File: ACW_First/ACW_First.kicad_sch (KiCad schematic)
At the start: 18 parts, among them J1 Screw_Terminal_01x02, J10 Conn_01x04_Pin, J11 24VDC, J12 Conn_01x02_Pin, J13 Conn_01x04_Socket, J14 Conn_01x02_Pin, J2 Conn_01x03_Pin, J3 3.8VDC, J4 5VDC, J5 12VDC, J6 Screw_Terminal_01x02, J7 Screw_Terminal_01x04, J8 Conn_01x02_Pin, J9 Conn_01x03_Socket

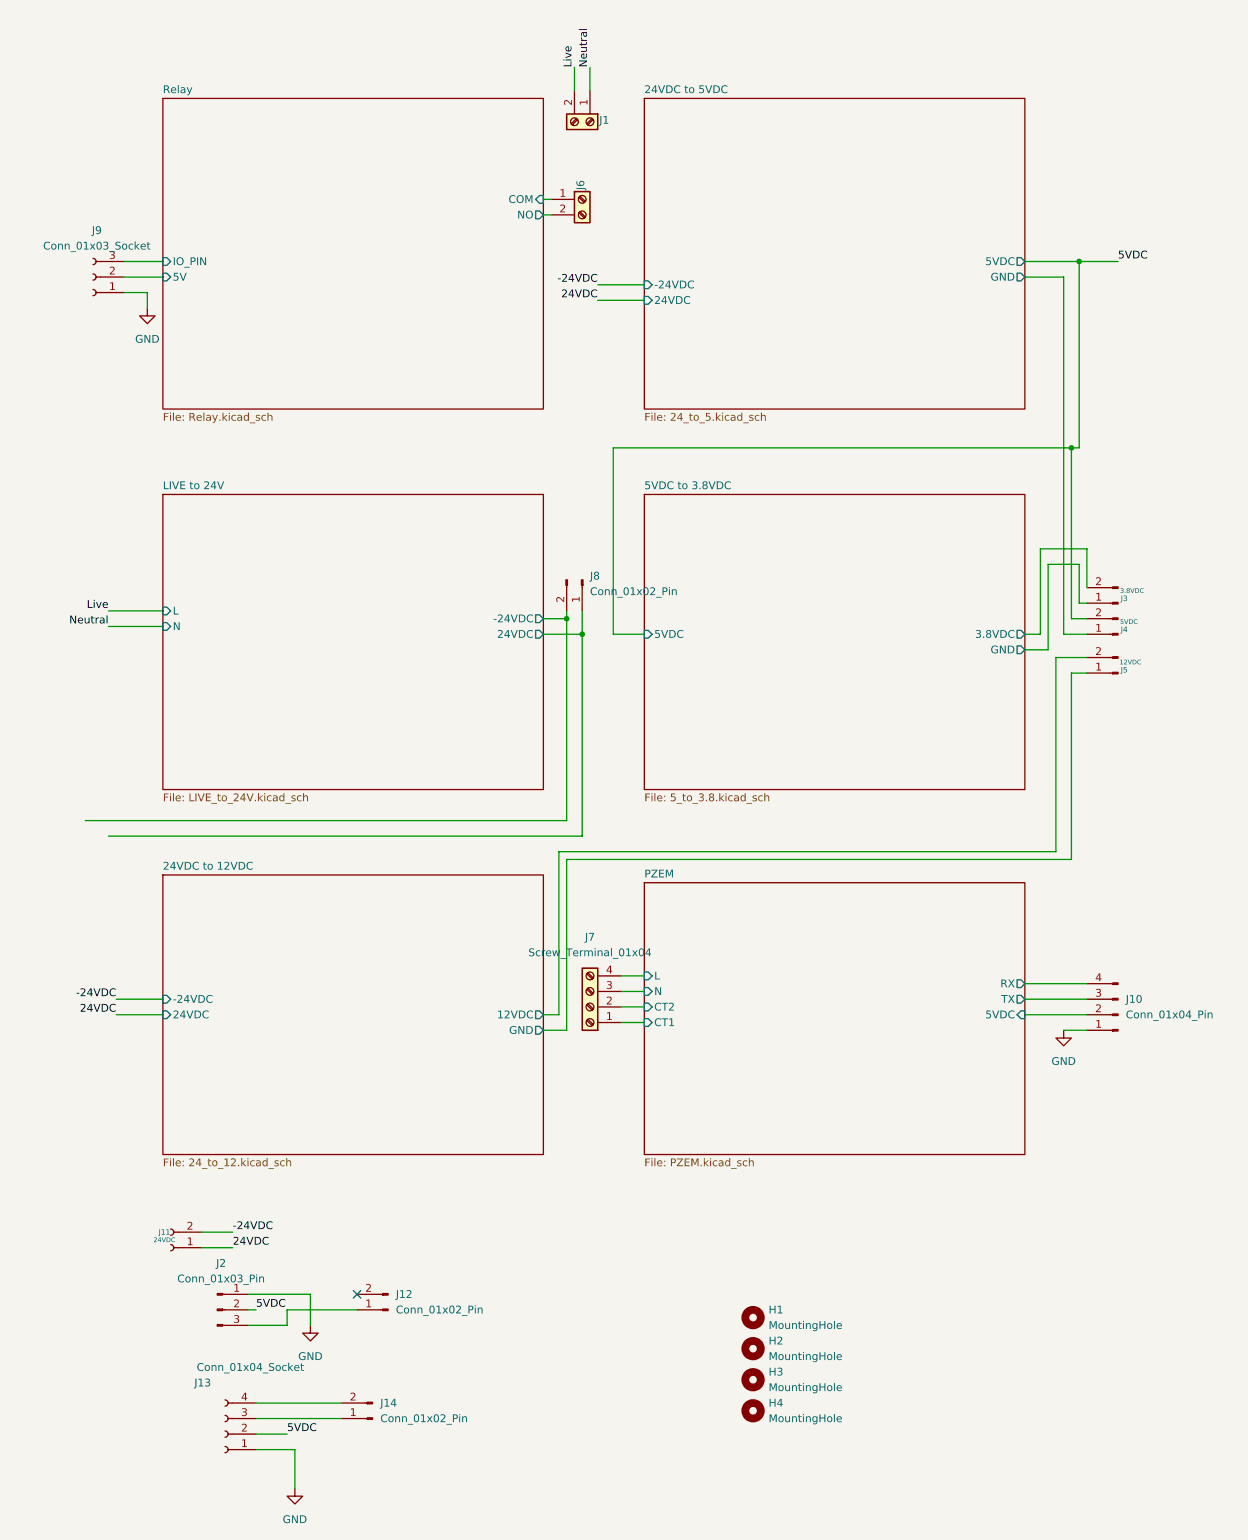
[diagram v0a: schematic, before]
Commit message: okokok
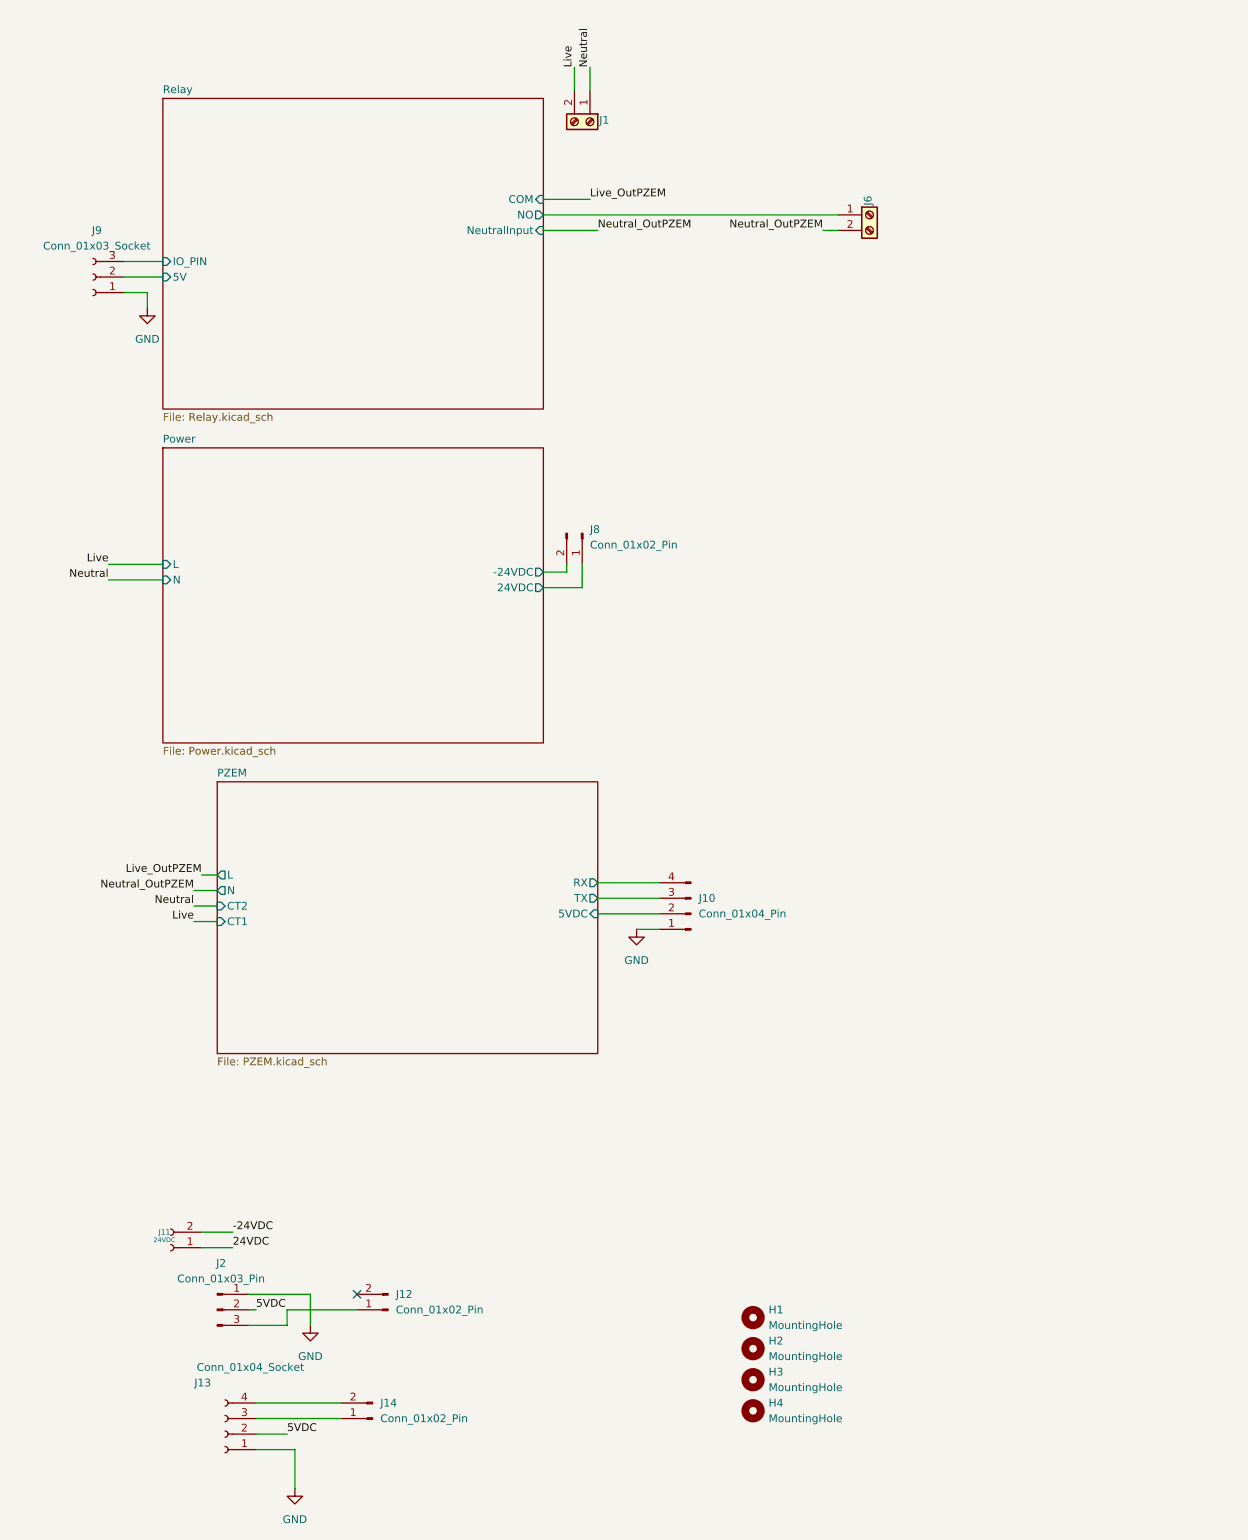
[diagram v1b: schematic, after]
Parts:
- removed J3: 3.8VDC, Connector_PinHeader_2.54mm:PinHeader_1x02_P2.54mm_Vertical, symbol Connector:Conn_01x02_Pin
- removed J4: 5VDC, Connector_PinHeader_2.54mm:PinHeader_1x02_P2.54mm_Vertical, symbol Connector:Conn_01x02_Pin
- removed J5: 12VDC, Connector_PinHeader_2.54mm:PinHeader_1x02_P2.54mm_Vertical, symbol Connector:Conn_01x02_Pin
- removed J7: Screw_Terminal_01x04, TerminalBlock_MetzConnect:TerminalBlock_MetzConnect_Type101_RT01604HBWC_1x04_P5.08mm_Horizontal, symbol Connector:Screw_Terminal_01x04
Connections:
- net Relay/COM is gone; now on net Relay/NO: J6.1 (Pin_1)
- net Relay/NO: no longer J6.2 (Pin_2)
- new net Neutral_OutPZEM: J6.2 (Pin_2)
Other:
- sheet LIVE to 24V renamed Power
- removed sheet 24VDC to 12VDC
- removed sheet 24VDC to 5VDC
- removed sheet 5VDC to 3.8VDC
- sheet Power: file LIVE_to_24V.kicad_sch -> Power.kicad_sch
- sheet Relay ports: added NeutralInput; removed none
- moved on the sheet: J10, J6, J8

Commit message: revisi
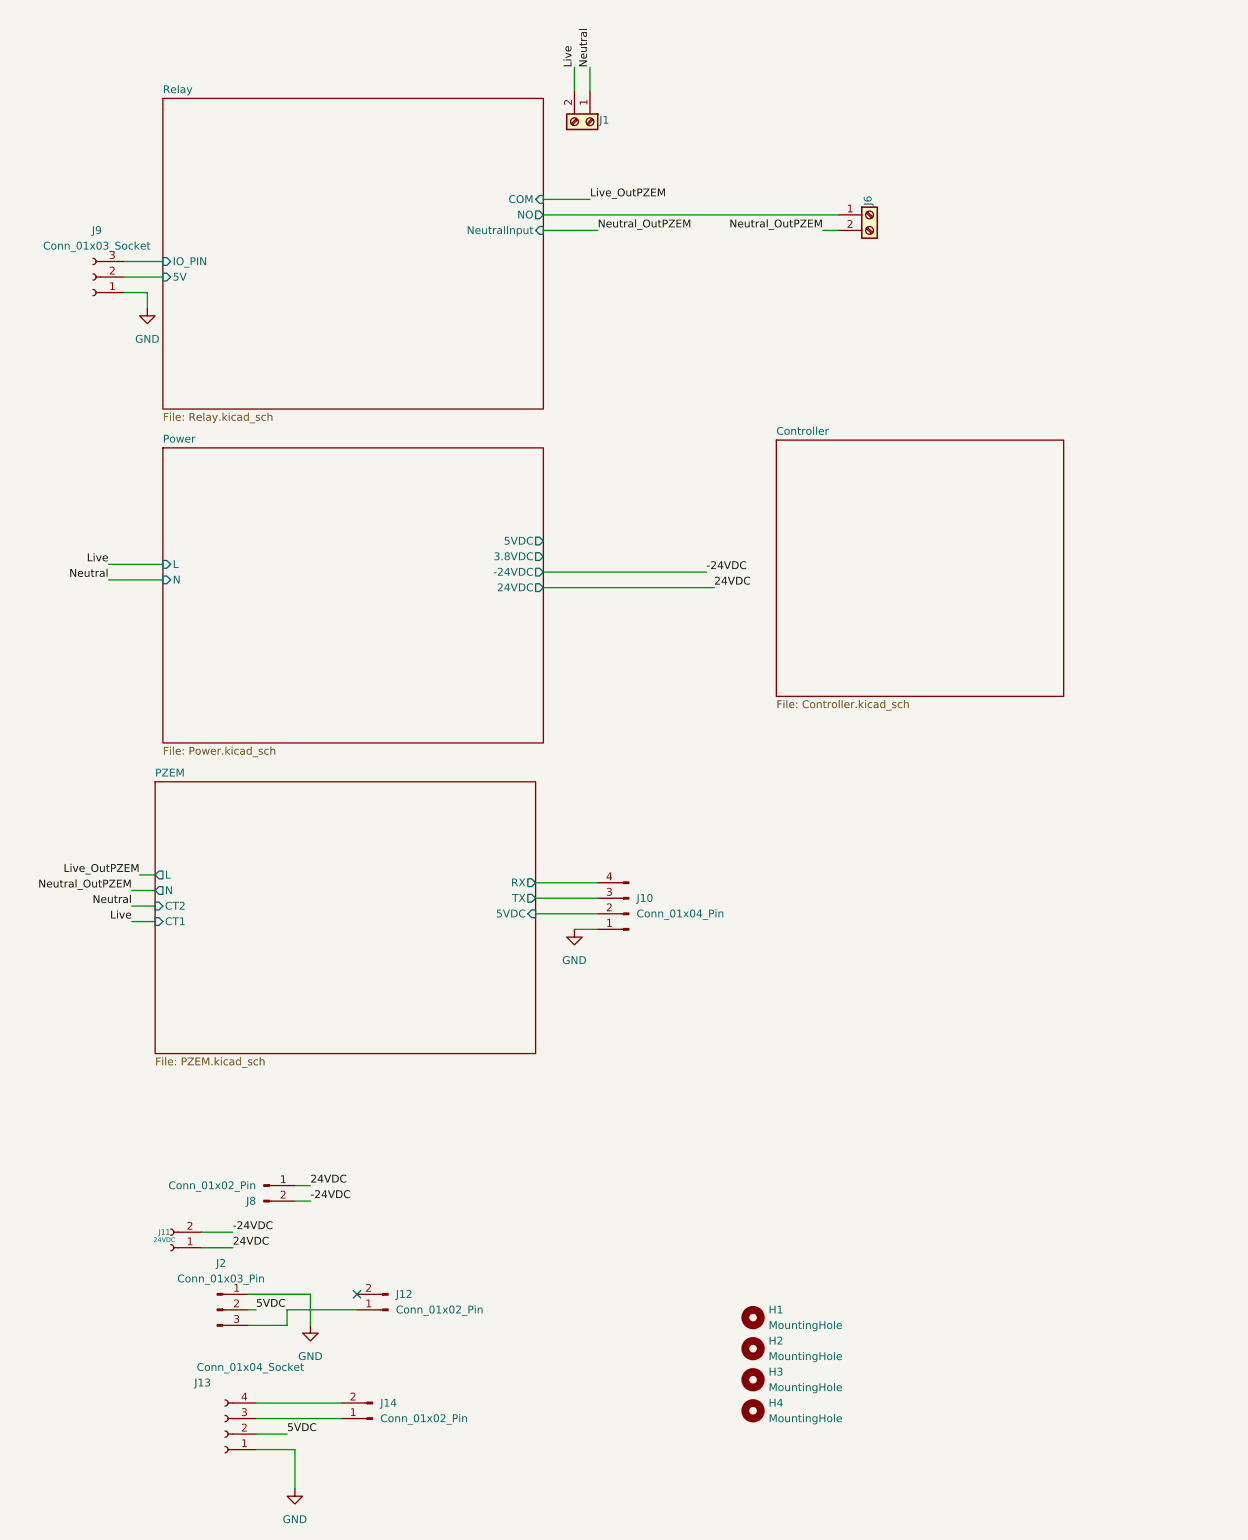
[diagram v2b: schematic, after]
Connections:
- net Power/-24VDC is gone; now on net -24VDC: J8.2 (Pin_2)
- net Power/24VDC is gone; now on net 24VDC: J8.1 (Pin_1)
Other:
- added sheet Controller (Controller.kicad_sch)
- sheet Power ports: added 3.8VDC, 5VDC; removed none
- moved on the sheet: J10, J8
